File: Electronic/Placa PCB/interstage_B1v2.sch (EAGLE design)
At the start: 8 parts, among them Q1 PMV16XNR, T5 MCP9808T-E/MS, T6 MCP9808T-E/MS

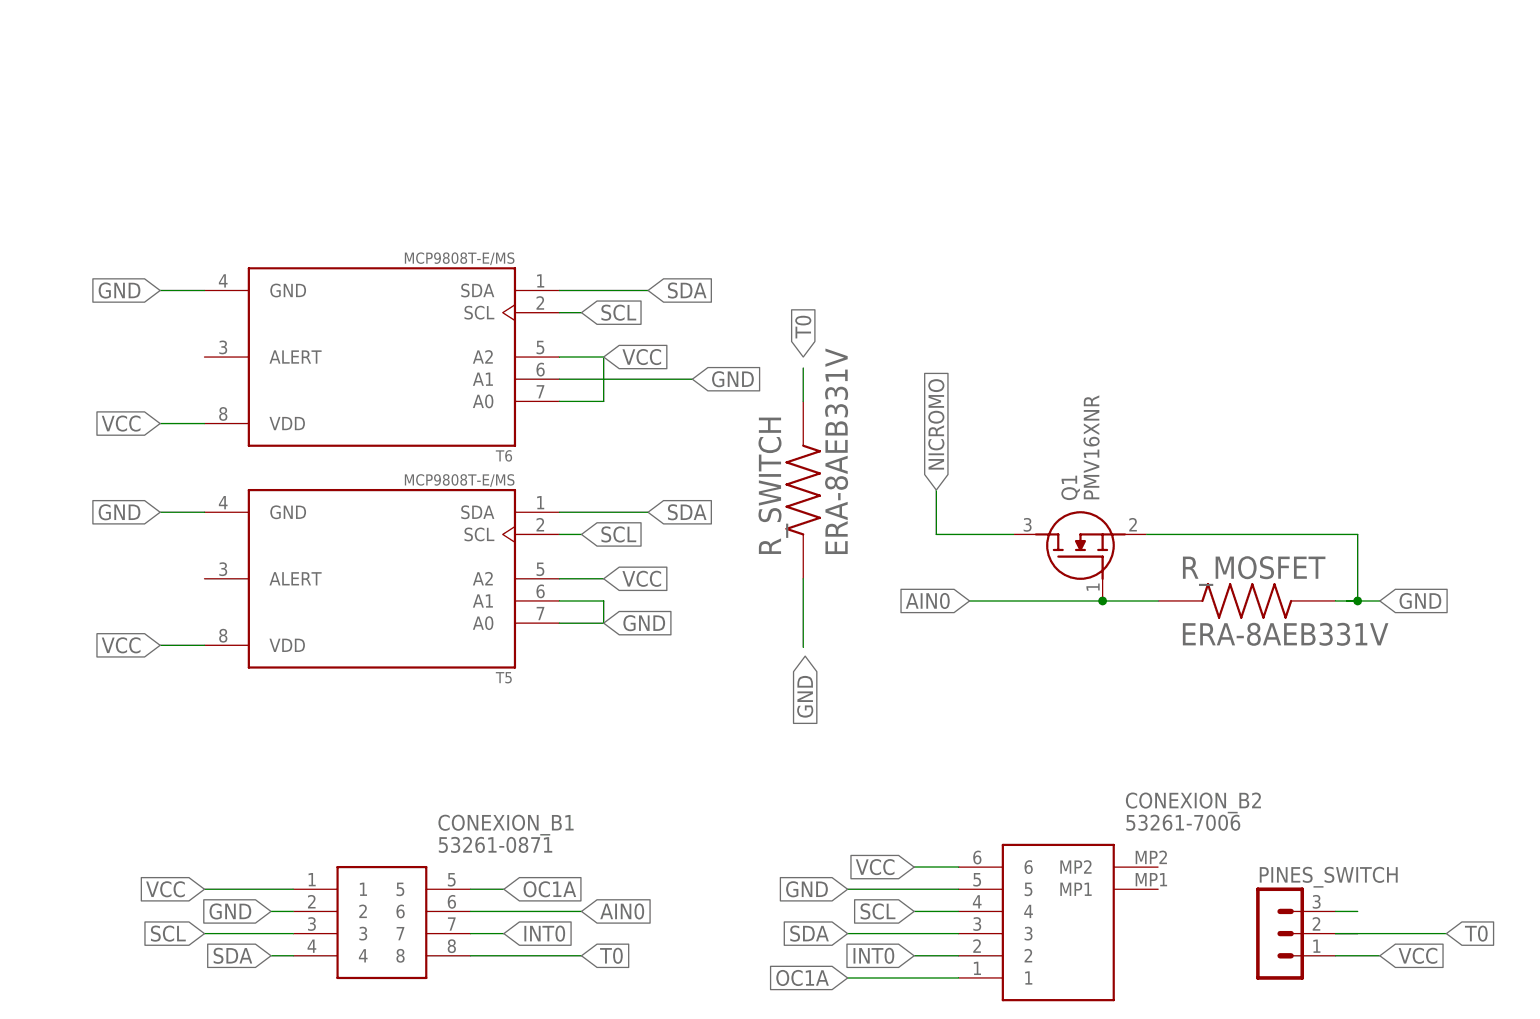
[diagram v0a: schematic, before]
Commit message: Avance
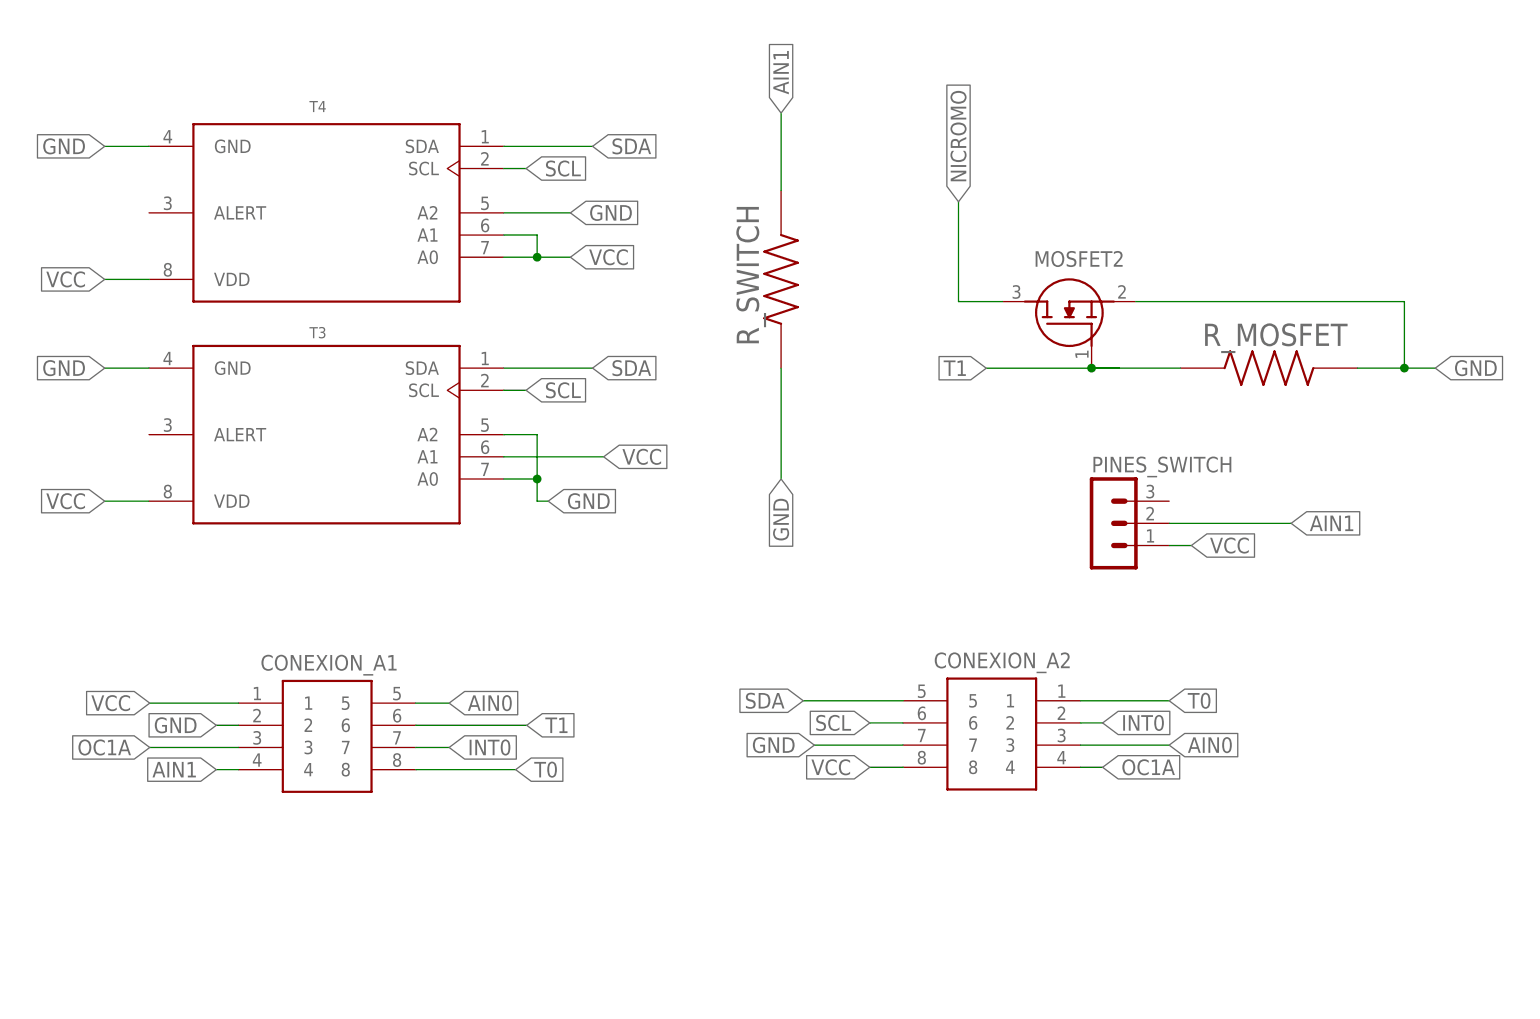
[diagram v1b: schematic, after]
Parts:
- removed CONEXION_B1: 53261-0871, SamacSys_Parts:53261-0871
- removed CONEXION_B2: 53261-7006, SamacSys_Parts:53261-7006
- removed Q1: PMV16XNR, SamacSys_Parts:PMV16XNR
- removed T5, T6: MCP9808T-E/MS, sensorSPEL:MCP9808T-E/MS
- added CONEXION_A1, CONEXION_A2: 53261-0871, SamacSys_Parts:53261-0871
- added MOSFET2: PMV16XNR, SamacSys_Parts:PMV16XNR
- added T3, T4: MCP9808T-E/MS, sensorSPEL:MCP9808T-E/MS
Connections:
- removed net N$7: PINES_SWITCH.3
- new net AIN1: CONEXION_A1.4, PINES_SWITCH.2, R_SWITCH.2
- new net T1: CONEXION_A1.6, MOSFET2.G, R_MOSFET.1
- net AIN0: now also CONEXION_A1.5, CONEXION_A2.3; no longer CONEXION_B1.6, Q1.G, R_MOSFET.1
- net GND: now also CONEXION_A1.2, CONEXION_A2.7, MOSFET2.S, T3.A0, T3.A2, T3.GND, T4.A2, T4.GND; no longer CONEXION_B1.2, CONEXION_B2.5, Q1.S, T5.A0, T5.A1, T5.GND, T6.A1, T6.GND
- net INT0: now also CONEXION_A1.7, CONEXION_A2.2; no longer CONEXION_B1.7, CONEXION_B2.2
- net NICROMO: now also MOSFET2.D; no longer Q1.D
- net OC1A: now also CONEXION_A1.3, CONEXION_A2.4; no longer CONEXION_B1.5, CONEXION_B2.1
- net SCL: now also CONEXION_A2.6, T3.SCL, T4.SCL; no longer CONEXION_B1.3, CONEXION_B2.4, T5.SCL, T6.SCL
- net SDA: now also CONEXION_A2.5, T3.SDA, T4.SDA; no longer CONEXION_B1.4, CONEXION_B2.3, T5.SDA, T6.SDA
- net T0: now also CONEXION_A1.8, CONEXION_A2.1; no longer CONEXION_B1.8, PINES_SWITCH.2, R_SWITCH.2
- net VCC: now also CONEXION_A1.1, CONEXION_A2.8, T3.A1, T3.VDD, T4.A0, T4.A1, T4.VDD; no longer CONEXION_B1.1, CONEXION_B2.6, T5.A2, T5.VDD, T6.A0, T6.A2, T6.VDD
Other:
- moved on the sheet: PINES_SWITCH, R_MOSFET, R_SWITCH
